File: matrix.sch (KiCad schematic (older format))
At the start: 180 parts

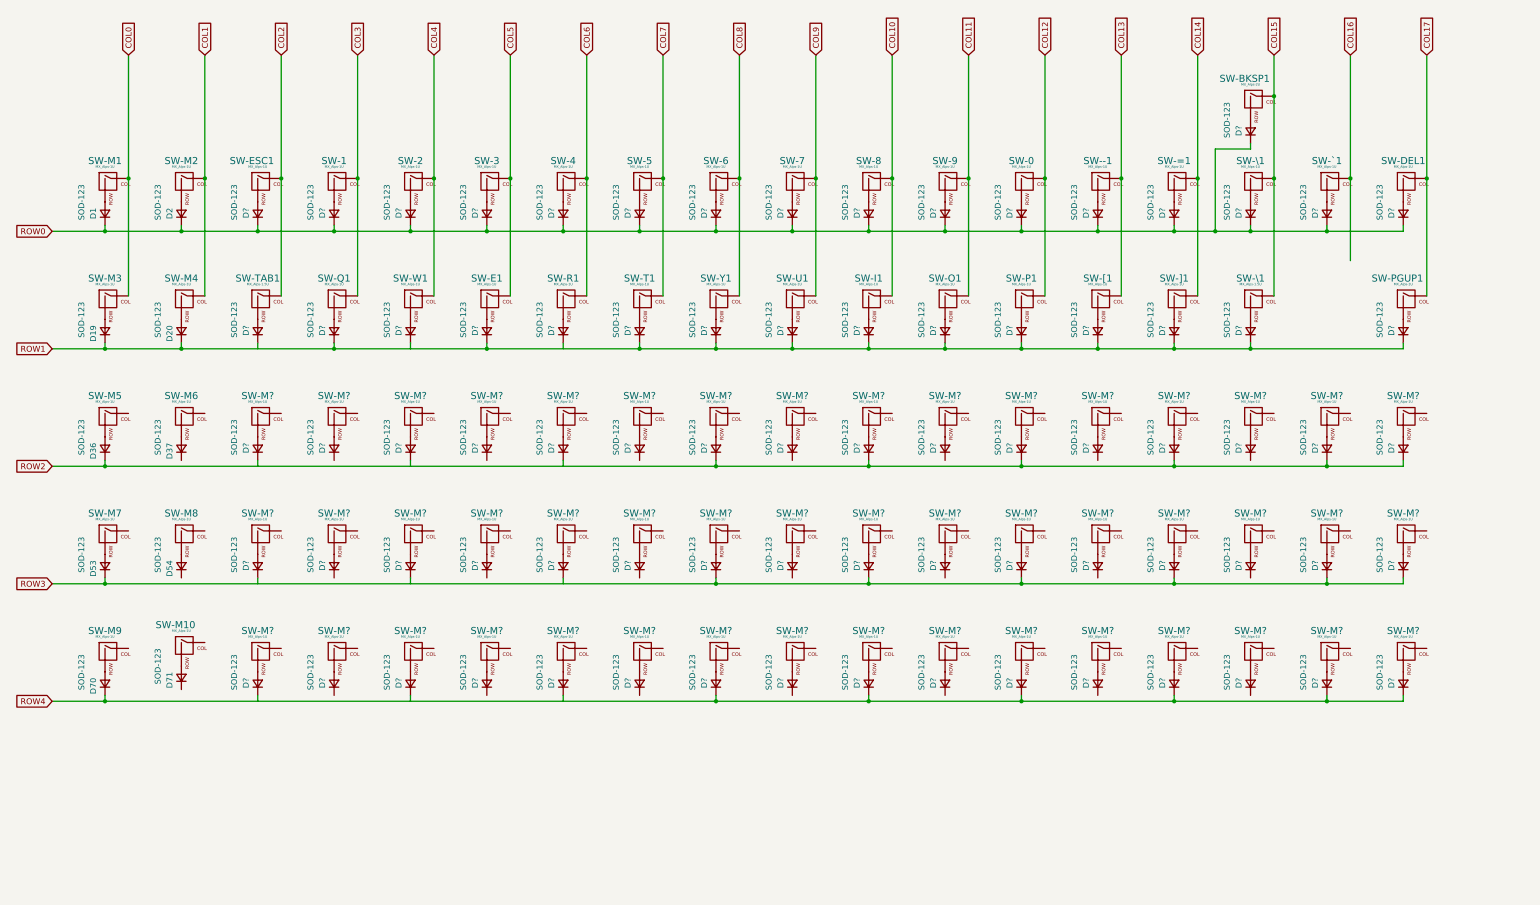
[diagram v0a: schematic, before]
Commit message: Matrix work
Additional work on the switch matrix.
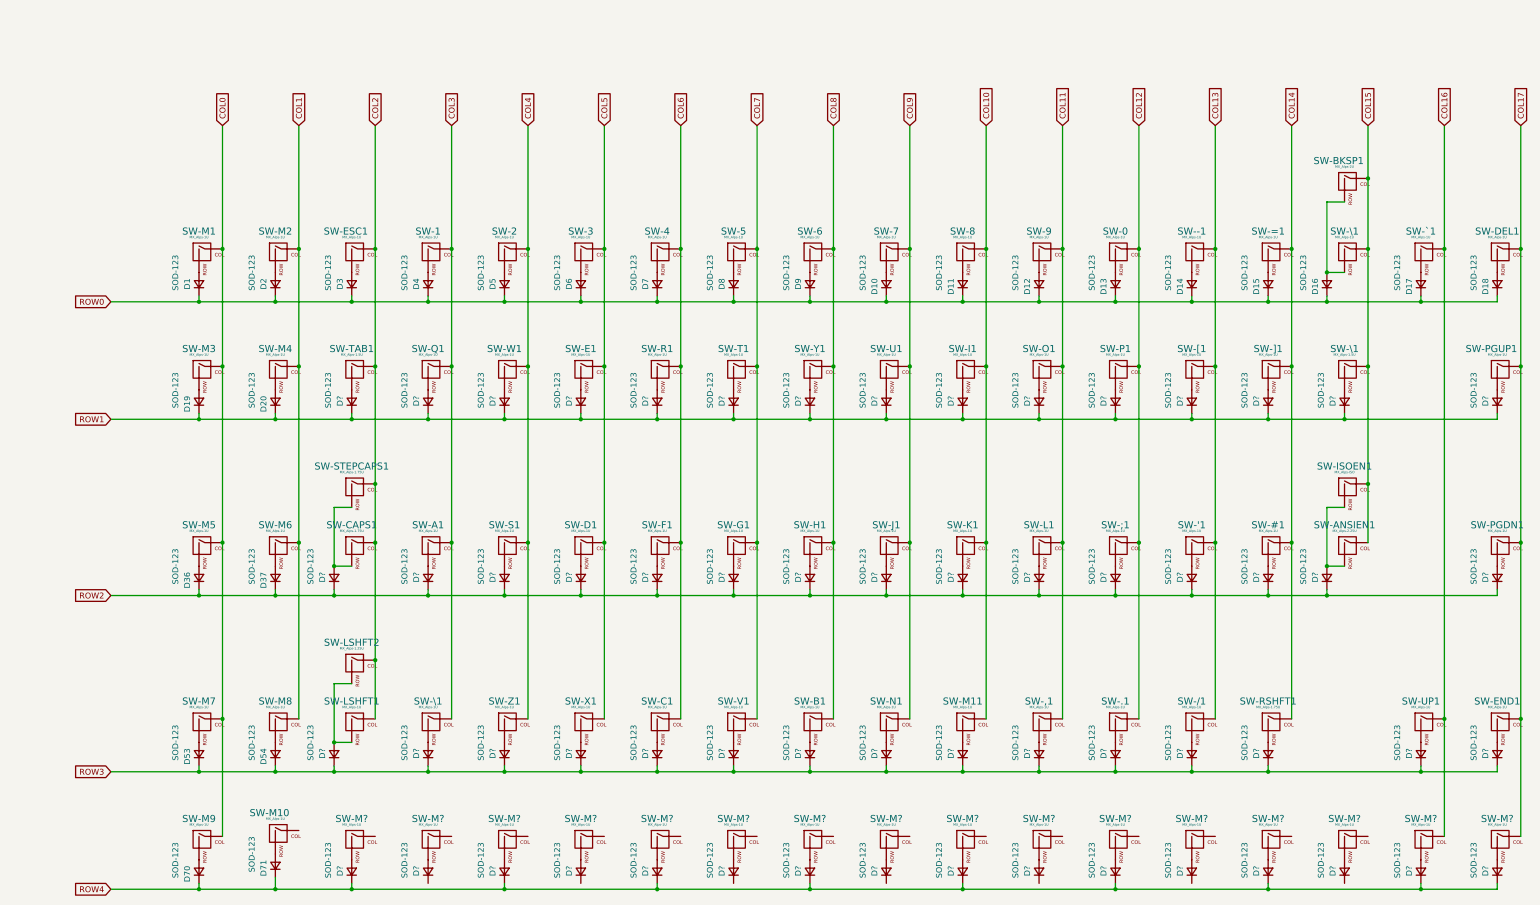
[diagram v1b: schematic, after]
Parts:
- removed D? (x3): SOD-123, Diode_SMD:D_SOD-123, symbol Device:D_Small
- removed SW-M? (x2): MX_Alps-1U, MX_Alps_Hybrid:MX-1U-NoLED, symbol MX_Alps_Hybrid:MX-NoLED
- added SW-ISOEN1: MX_Alps-ISO, MX_Alps_Hybrid:MX-ISO-ReversedStabilizers, symbol MX_Alps_Hybrid:MX-NoLED
- added SW-LSHFT2: MX_Alps-1.25U, MX_Alps_Hybrid:MX-1.25U-NoLED, symbol MX_Alps_Hybrid:MX-NoLED
- added SW-STEPCAPS1: MX_Alps-1.75U, MX_Alps_Hybrid:MX-1.75U-NoLED, symbol MX_Alps_Hybrid:MX-NoLED
- SW-ANSIEN1: renamed from SW-M?; value MX_Alps-1U -> MX_Alps-2.25U; footprint MX_Alps_Hybrid:MX-1U-NoLED -> MX_Alps_Hybrid:MX-2.25U-NoLED
- SW-CAPS1, SW-RSHFT1: renamed from SW-M?; value MX_Alps-1U -> MX_Alps-1.75U; footprint MX_Alps_Hybrid:MX-1U-NoLED -> MX_Alps_Hybrid:MX-1.75U-NoLED
- SW-LSHFT1: renamed from SW-M?; footprint MX_Alps_Hybrid:MX-1U-NoLED -> MX_Alps_Hybrid:MX-2.25U-NoLED
- gave numbers to parts that had none: 42
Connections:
- wire segments 159 -> 248
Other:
- moved on the sheet: D1, D10, D11, D12, D13, D14, D15, D16, D17, D18, D19, D2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
